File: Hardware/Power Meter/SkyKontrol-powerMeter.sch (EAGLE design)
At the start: 23 parts, among them J4 SBH11-PBPC-D05, T1 MMBT3904, T2 MMBT3904, U1 PIC12F1822-E/SN

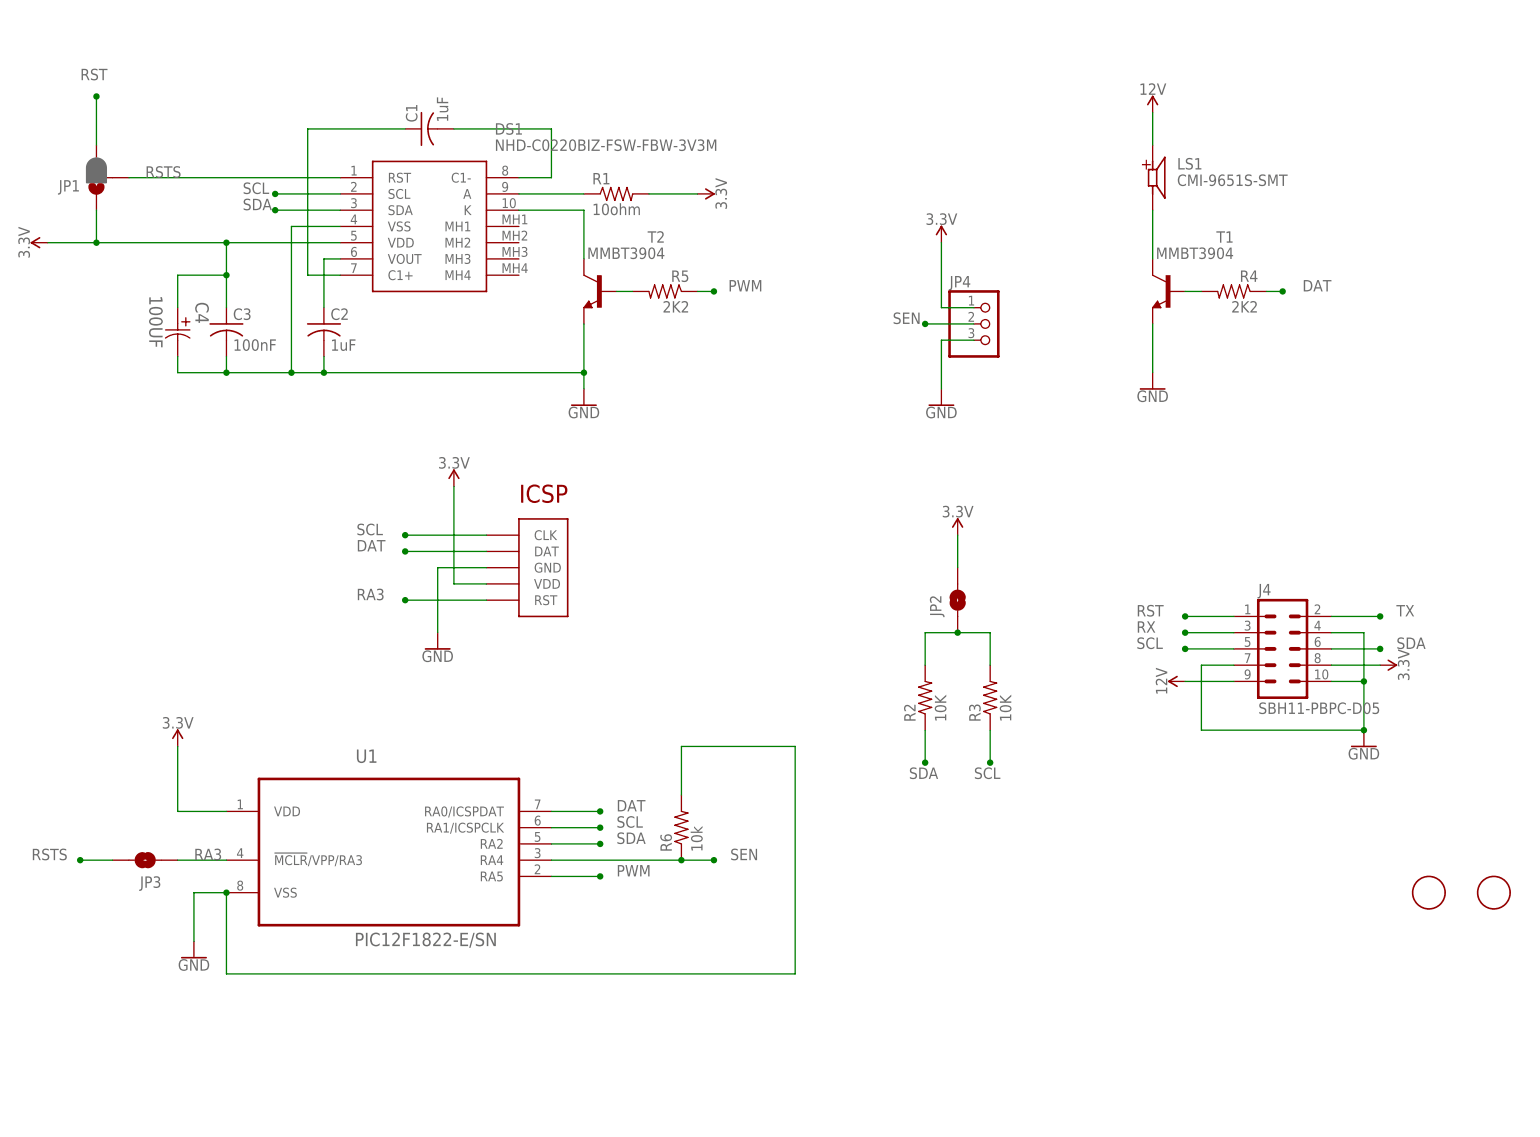
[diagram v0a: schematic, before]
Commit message: documentation add
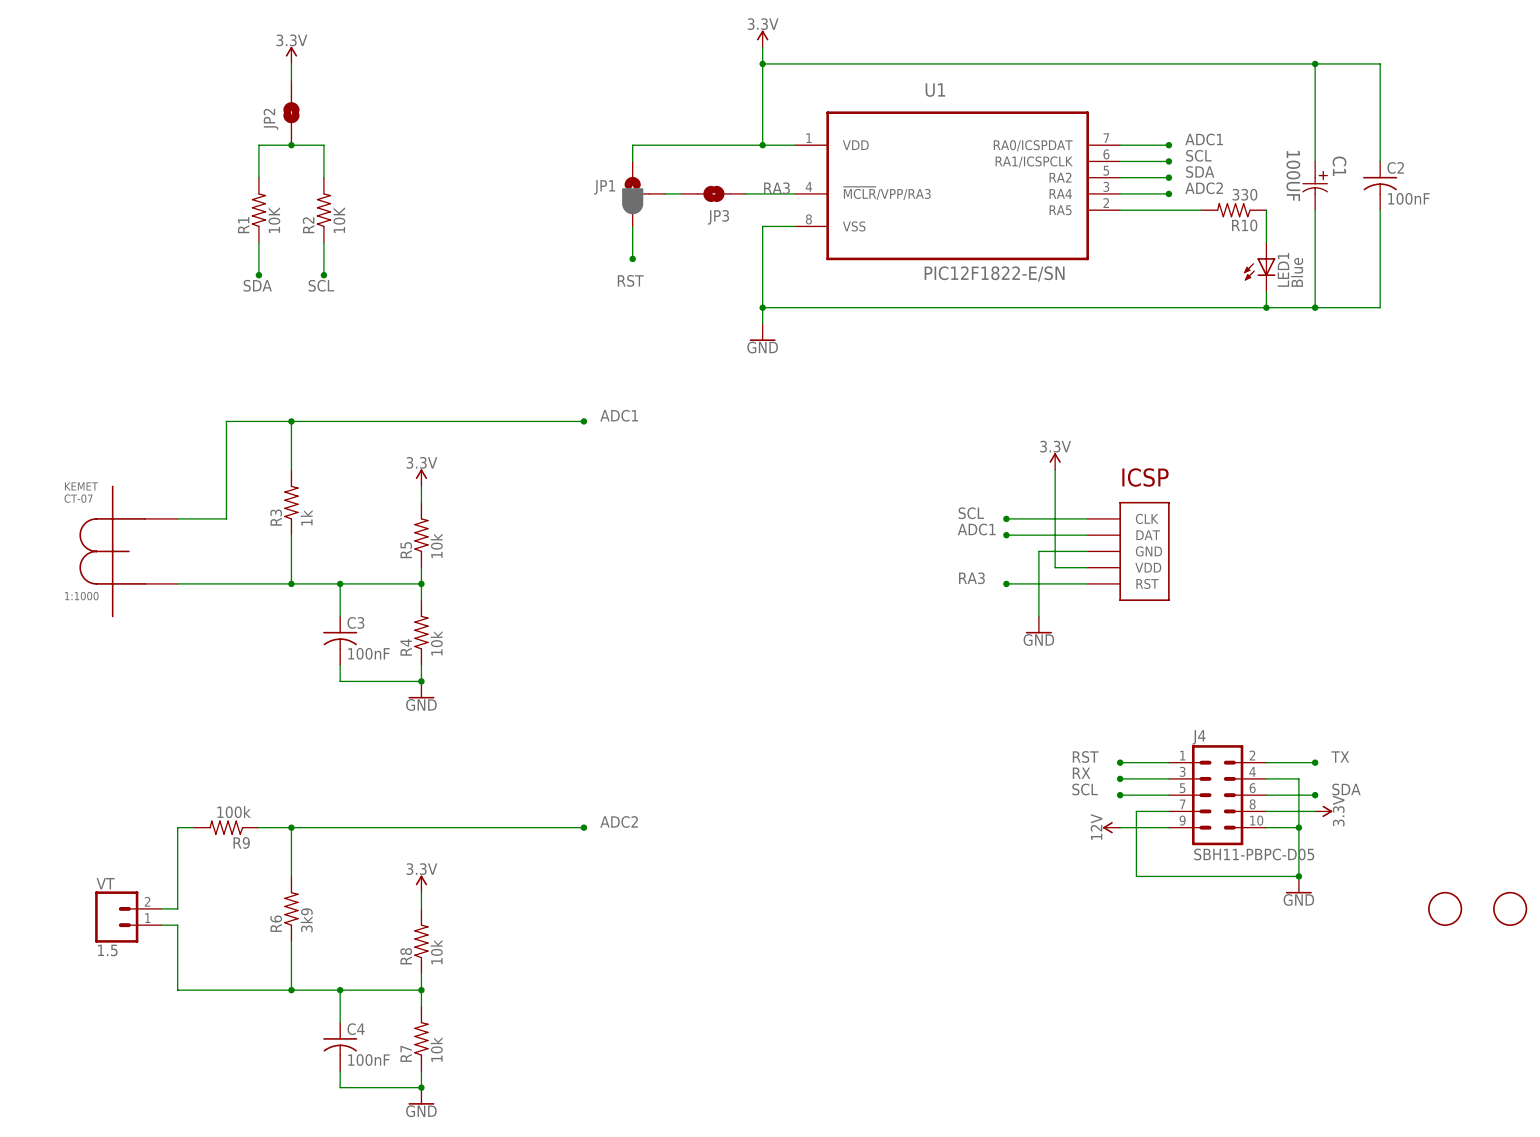
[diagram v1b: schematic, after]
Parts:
- removed DS1: NHD-C0220BIZ-FSW-FBW-3V3M, NHD-C0220BIZ-FSW-FBW-3V3M:NHD-C0220BIZ-FSW-FBW-3V3M
- removed JP4: (no value), adafruit:PINHD-1X3CB
- removed LS1: CMI-9651S-SMT, CMI-9651S-SMT:CMI-9651S-SMT
- removed T1, T2: MMBT3904, transistor:MMBT3904LT1-NPN-SOT23-BEC
- added LED1: Blue, adafruit:LEDCHIPLED_1206
- added R10: 330, adafruit:R-US_R0805
- added R7, R8: 10k, adafruit:R-US_R0805
- added R9: 100k, adafruit:R-US_R0805
- added U$4: CT-07KEMET, CT-07:CT-07KEMET
- added VT: 1.5, SparkFun-Connectors:CONN_025MM
- C1: value 1uF -> 100UF; device adafruit:C-USC0603K -> Panasonic-EEEFT_EEEH:EEE-HA1E101XP-CASE-D8
- C2: value 1uF -> 100nF
- C4: value 100UF -> 100nF; device Panasonic-EEEFT_EEEH:EEE-HA1E101XP-CASE-D8 -> adafruit:C-USC0603K
- R1: value 10ohm -> 10K
- R3: value 10K -> 1k
- R4, R5: value 2K2 -> 10k
- R6: value 10k -> 3k9
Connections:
- removed net DAT: R4.1, U$2.DAT, U1.RA0/ICSPDAT
- removed net N$12: R4.2, T1.B
- removed net N$17: DS1.K, T2.C
- removed net N$19: R5.2, T2.B
- removed net PWM: R5.1, U1.RA5
- removed net RSTS: DS1.RST, JP1.2, JP3.2
- removed net SEN: JP4.2, R6.1, U1.RA4
- new net ADC1: R3.2, U$2.DAT, U$4.C1, U1.RA0/ICSPDAT
- new net ADC2: R6.2, R9.1, U1.RA4
- new net N$9: R10.2, U1.RA5
- net 12V: no longer LS1.P
- net 3.3V: now also C1.1, C2.1, R5.2, R8.2; no longer C3.1, C4.1, DS1.VDD, JP4.1, R1.2
- net GND: now also C1.2, LED1.C, R4.1, R7.1; no longer DS1.VSS, JP4.3, R6.2, T1.E, T2.E
- net N$1: now also JP1.2, JP3.2; no longer C2.1, DS1.VOUT
- net N$10: now also LED1.A, R10.1; no longer LS1.N, T1.C
- net N$2: now also C3.1, R3.1, R4.2, R5.1, U$4.C2; no longer C1.2, DS1.C1-
- net N$3: now also R9.2, VT.2; no longer C1.1, DS1.C1+
- net N$4: now also C4.1, R6.1, R7.2, R8.1, VT.1; no longer DS1.A, R1.1
- net N$8: now also R1.2; no longer R3.2
- net SCL: now also R2.1; no longer DS1.SCL, R3.1
- net SDA: now also R1.1; no longer DS1.SDA, R2.1
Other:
- moved on the sheet: C2, C3, J4, JP1, JP2, JP3, R1, R2, R3, R4, R5, R6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
